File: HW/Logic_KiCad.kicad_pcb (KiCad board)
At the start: 2 copper layers, 152 parts, among them J1 USB_B_Micro, Q1 Q_NPN_BCE, Q2 Q_NPN_BCE, Q3 Q_PMOS_DGS, Q4 Q_PMOS_DGS, Q7 Q_PMOS_DGS, SW1 SW_SPDT, SW10 button, SW11 button, SW12 button, SW2 button, SW3 button, SW4 button, SW5 button, SW6 button, SW7 button, SW8 button, SW9 button, U1 ESP32-PICO-D4, U2 CP2102N-A01-GQFN28, U3 SY8105, U4 Dual_battery, U5 TP4056

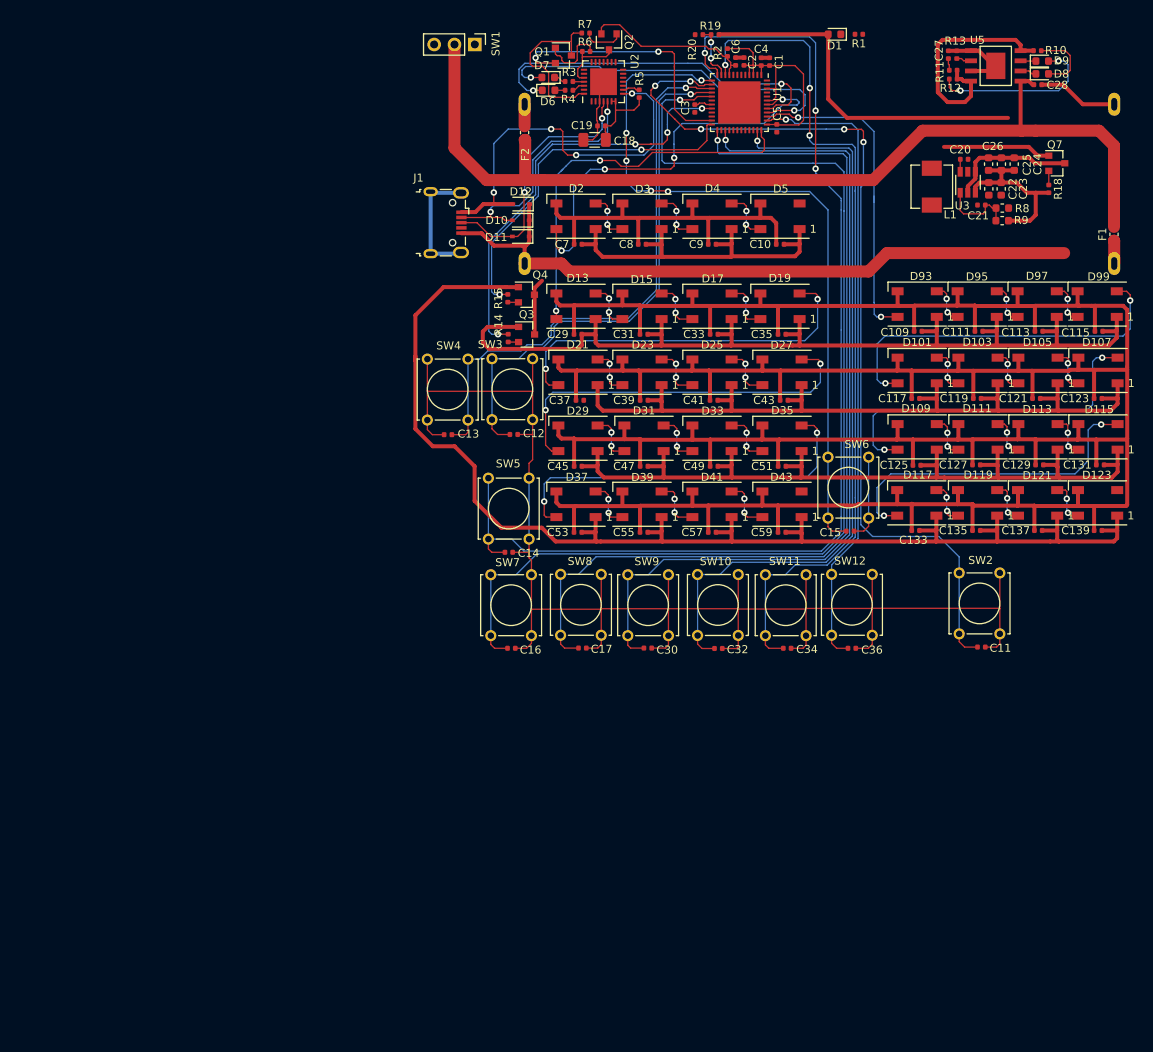
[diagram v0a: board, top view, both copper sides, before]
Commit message: finishing routing, make fab
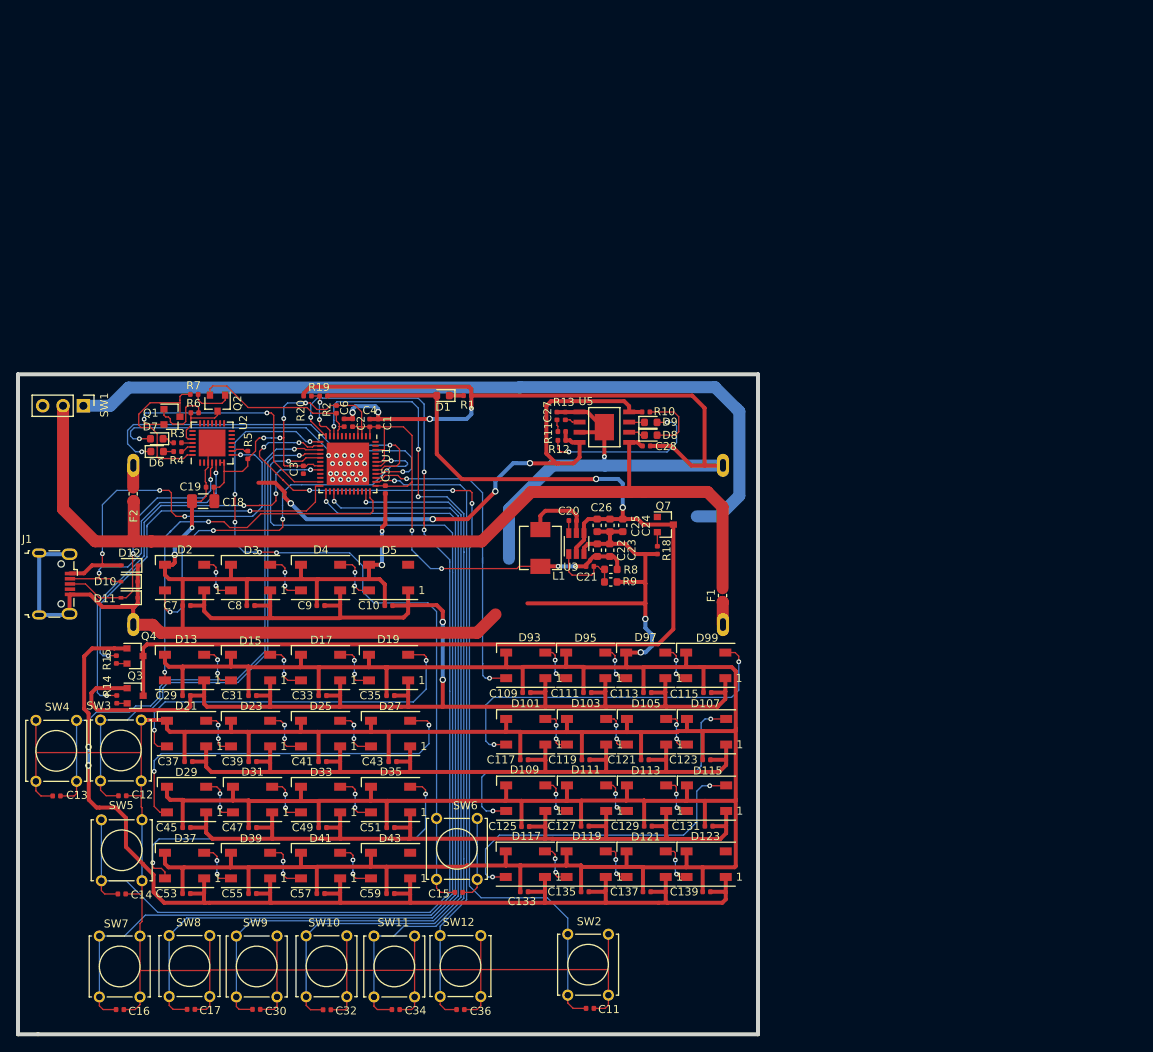
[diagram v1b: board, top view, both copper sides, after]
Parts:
- moved C15 66.6 mm to (140.1, 124.8)
- moved SW11 66.6 mm to (129.5, 137.8)
- moved SW2 66.6 mm to (153.7, 137.6)
- moved SW6 66.6 mm to (137.3, 123.1)
- moved C109 66.6 mm to (148.6, 99.8)
- moved C11 66.6 mm to (156.5, 139.3)
- moved C111 66.6 mm to (156.2, 99.8)
- moved C113 66.6 mm to (163.7, 99.8)
- moved C115 66.6 mm to (171.2, 99.8)
- moved C119 66.6 mm to (156.0, 108.2)
- moved C12 66.6 mm to (98.0, 112.7)
- moved C121 66.6 mm to (163.4, 108.2)
- moved C123 66.6 mm to (171.1, 108.2)
- moved C125 66.6 mm to (148.4, 116.5)
- moved C127 66.6 mm to (155.9, 116.5)
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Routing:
- net GND: track 876.0 -> 1030.6 mm, vias 0 -> 31
- net V_BAT_SPINANE: track 13.6 -> 101.2 mm
- net V_BAT: track 68.3 -> 152.4 mm, vias 0 -> 2
- net +3V3: track 46.4 -> 107.5 mm, vias 0 -> 8
- net VBUS: track 77.1 -> 120.6 mm, vias 4 -> 8
- net V_BAT_1: track 384.6 -> 402.9 mm, vias 0 -> 2
- net V_BAT_2: track 166.0 -> 153.1 mm, vias 0 -> 2
- net Net-(C20-Pad1): track 0.00 -> 8.98 mm
- net Net-(D1-Pad1): track 0.00 -> 1.78 mm
- net BARVA_2: track 115.3 -> 114.4 mm
- net IO0: track 33.4 -> 32.6 mm
- net BARVA_5: track 105.9 -> 105.2 mm
- net BTN_SIPKA_VPRAVO: track 92.7 -> 92.1 mm
- net BARVA_4: track 94.6 -> 94.1 mm
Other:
- board outline added: 92.5 x 82.5 mm
- rule trace_min: 0.09 -> 0.127
- rule via_min_drill: 0.3 -> 0.2
- rule via_min_size: 0.4 -> 0.45
